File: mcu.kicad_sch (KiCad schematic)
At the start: 38 parts, among them IC1 MAX98357AETE+T, IC2 MAX98357AETE+T, SW1 SW_Push, U1 STM32WB55CGU6, Y1 32MHz, Y2 32KHz768

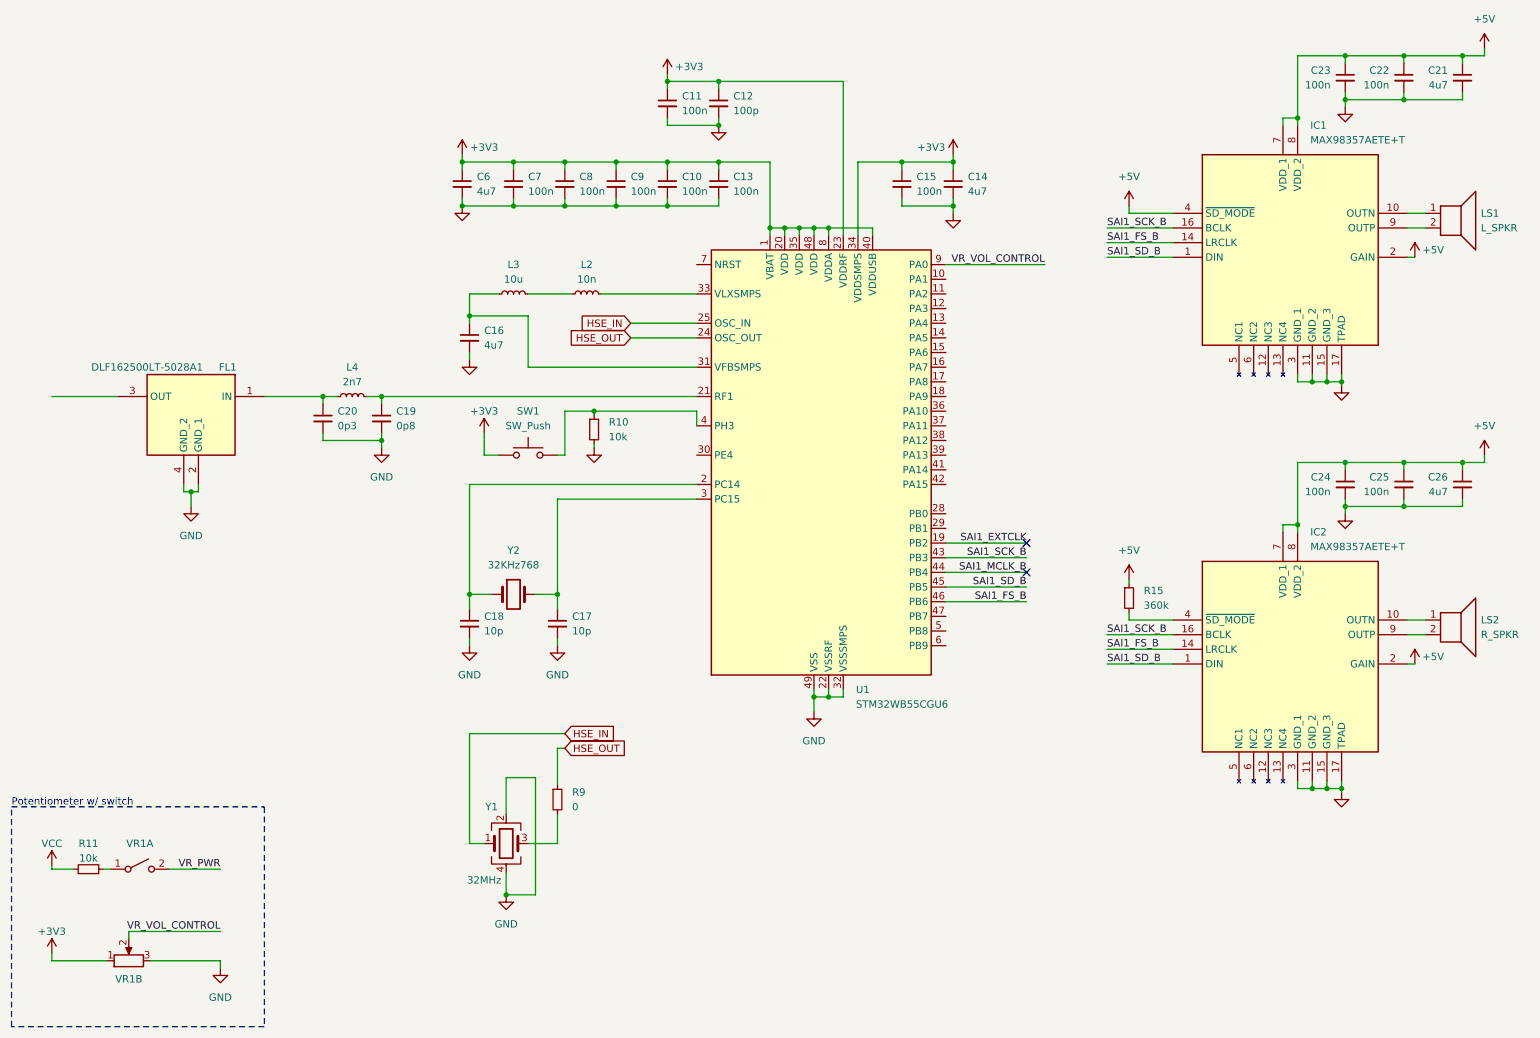
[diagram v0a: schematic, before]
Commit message: Finished rev 1 of the board
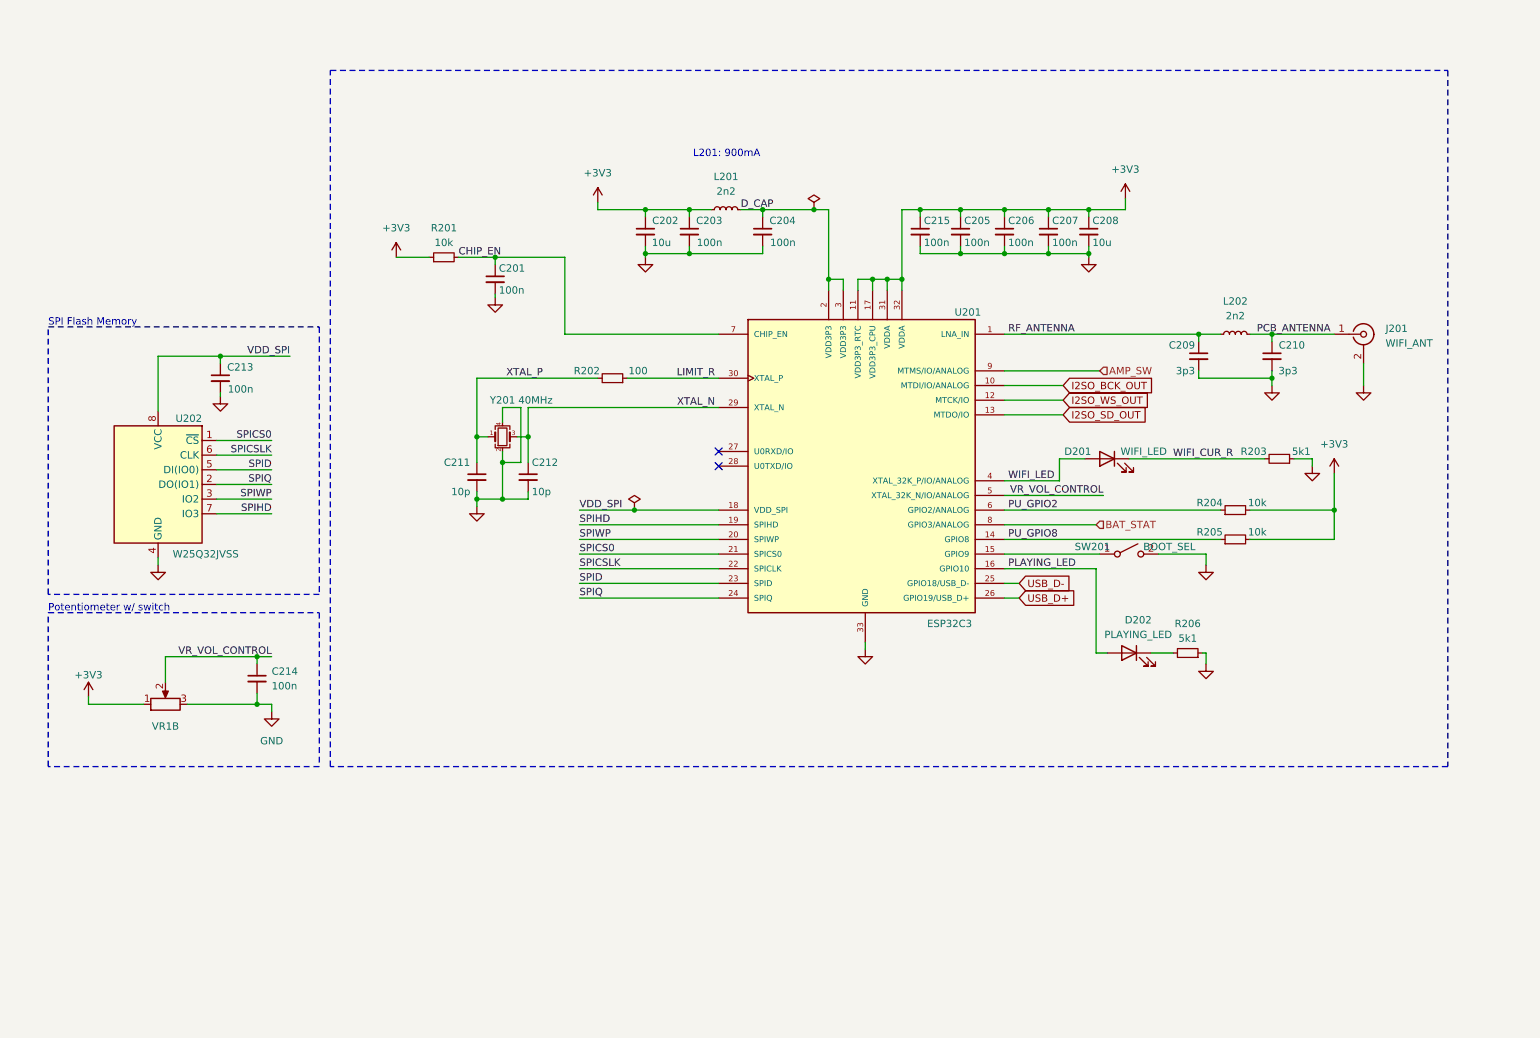
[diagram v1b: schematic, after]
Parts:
- removed C10, C11, C13, C15, C22, C23, C24, C25, C7, C8, C9: 100n, symbol Device:C_Small
- removed C12: 100p, symbol Device:C_Small
- removed C14, C16, C21, C26, C6: 4u7, symbol Device:C_Small
- removed C17, C18: 10p, symbol Device:C_Small
- removed C19: 0p8, symbol Device:C_Small
- removed C20: 0p3, symbol Device:C_Small
- removed FL1: DLF162500LT-5028A1, DLF162500LT5028A1, symbol custom_library:DLF162500LT-5028A1
- removed IC1, IC2: MAX98357AETE+T, QFN50P300X300X80-17N, symbol custom_library:MAX98357AETE+T
- removed L2: 10n, symbol Device:L_Small
- removed L3: 10u, symbol Device:L_Small
- removed L4: 2n7, symbol Device:L_Small
- removed LS1: L_SPKR, symbol Device:Speaker
- removed LS2: R_SPKR, symbol Device:Speaker
- removed R10, R11: 10k, symbol Device:R_Small
- removed R15: 360k, symbol Device:R_Small
- removed R9: 0, symbol Device:R_Small
- removed SW1: SW_Push, symbol Switch:SW_Push
- removed U1: STM32WB55CGU6, Package_DFN_QFN:QFN-48-1EP_7x7mm_P0.5mm_EP5.6x5.6mm, symbol MCU_ST_STM32WB:STM32WB55CGUx
- removed unit 1 of VR1
- removed Y1: 32MHz, symbol Device:Crystal_GND24
- removed Y2: 32KHz768, symbol Device:Crystal
- added C201, C203, C204, C205, C206, C207, C213, C214, C215: 100n, Capacitor_SMD:C_0402_1005Metric, symbol Device:C_Small
- added C202, C208: 10u, Capacitor_SMD:C_0603_1608Metric, symbol Device:C_Small
- added C209, C210: 3p3, Capacitor_SMD:C_0402_1005Metric, symbol Device:C_Small
- added C211, C212: 10p, Capacitor_SMD:C_0402_1005Metric, symbol Device:C_Small
- added D201: WIFI_LED, LED_SMD:LED_0603_1608Metric, symbol Device:LED
- added D202: PLAYING_LED, LED_SMD:LED_0603_1608Metric, symbol Device:LED
- added J201: WIFI_ANT, Connector_Coaxial:SMA_Amphenol_901-143_Horizontal, symbol Connector:Conn_Coaxial
- added L201, L202: 2n2, Inductor_SMD:L_0402_1005Metric, symbol Device:L_Small
- added R201, R204, R205: 10k, Resistor_SMD:R_0402_1005Metric, symbol Device:R_Small
- added R202: 100, Resistor_SMD:R_0402_1005Metric, symbol Device:R_Small
- added R203, R206: 5k1, Resistor_SMD:R_0402_1005Metric, symbol Device:R_Small
- added SW201: BOOT_SEL, Button_Switch_SMD:SW_SPST_SKQG_WithoutStem, symbol Switch:SW_SPST
- added U201: ESP32C3, Package_DFN_QFN:HVQFN-32-1EP_5x5mm_P0.5mm_EP3.1x3.1mm_ThermalVias, symbol ESP32C3:ESP32C3
- added U202: W25Q32JVSS, Package_SO:SOIC-8_5.23x5.23mm_P1.27mm, symbol Memory_Flash:W25Q32JVSS
- added Y201: 40MHz, Crystal:Crystal_SMD_3225-4Pin_3.2x2.5mm, symbol Device:Crystal_GND24_Small
- VR1: footprint (none) -> Internet_Radio_Speaker:Potentiometer_Alps_RK0971111Z1P; LCSC (none) -> C2687318
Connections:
- net +3V3: now also C202.1, C203.1, C205.1, C206.1, C207.1, C208.1, C215.1, L201.1, R201.1, R204.2, R205.2, U201.11 (VDD3P3_RTC), U201.17 (VDD3P3_CPU), U201.31 (VDDA), U201.32 (VDDA)
- net GND: now also C201.2, C202.2, C203.2, C204.2, C205.2, C206.2, C207.2, C208.2, C209.2, C210.2, C211.2, C212.2, C213.2, C214.2, C215.2, J201.2 (Ext), R203.1, R206.1, SW201.2 (B), U201.33 (GND), U202.4 (GND), Y201.2, Y201.4
- net VR_VOL_CONTROL: now also C214.1, U201.5 (XTAL_32K_N/IO/ANALOG)
- new net: D202.1 (K), R206.2
- new net: SW201.1 (A), U201.15 (GPIO9)
- new net AMP_SW: U201.9 (MTMS/IO/ANALOG)
- new net BAT_STAT: U201.8 (GPIO3/ANALOG)
- new net CHIP_EN: C201.1, R201.2, U201.7 (CHIP_EN)
- new net D_CAP: C204.1, L201.2, U201.2 (VDD3P3), U201.3 (VDD3P3)
- new net I2SO_BCK_OUT: U201.10 (MTDI/IO/ANALOG)
- new net I2SO_SD_OUT: U201.13 (MTDO/IO)
- new net I2SO_WS_OUT: U201.12 (MTCK/IO)
- new net LIMIT_R: R202.1, U201.30 (XTAL_P)
- new net PCB_ANTENNA: C210.1, J201.1 (In), L202.2
- new net PLAYING_LED: D202.2 (A), U201.16 (GPIO10)
- new net PU_GPIO2: R204.1, U201.6 (GPIO2/ANALOG)
- new net PU_GPIO8: R205.1, U201.14 (GPIO8)
- new net RF_ANTENNA: C209.1, L202.1, U201.1 (LNA_IN)
- new net SPICS0: U201.21 (SPICS0), U202.1 (~{CS})
- new net SPICSLK: U201.22 (SPICLK), U202.6 (CLK)
- new net SPID: U201.23 (SPID), U202.5 (DI(IO0))
- new net SPIHD: U201.19 (SPIHD), U202.7 (IO3)
- new net SPIQ: U201.24 (SPIQ), U202.2 (DO(IO1))
- new net SPIWP: U201.20 (SPIWP), U202.3 (IO2)
- new net USB_D+: U201.26 (GPIO19/USB_D+)
- new net USB_D-: U201.25 (GPIO18/USB_D-)
- new net VDD_SPI: C213.1, U201.18 (VDD_SPI), U202.8 (VCC)
- new net WIFI_CUR_R: D201.1 (K), R203.2
- new net WIFI_LED: D201.2 (A), U201.4 (XTAL_32K_P/IO/ANALOG)
- new net XTAL_N: C212.1, U201.29 (XTAL_N), Y201.3
- new net XTAL_P: C211.1, R202.2, Y201.1
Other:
- note added: "L201: 900mA"
- note added: "SPI Flash Memory"
- company: (none) -> ST
- title: (none) -> Internet Radio Speaker
- moved on the sheet: VR1B
